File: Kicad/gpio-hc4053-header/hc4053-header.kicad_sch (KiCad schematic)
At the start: 7 parts, among them K1 GPIO IN, K2 I/O, K3 I/O, U1 74HC4053, U2 3M-SJ5376

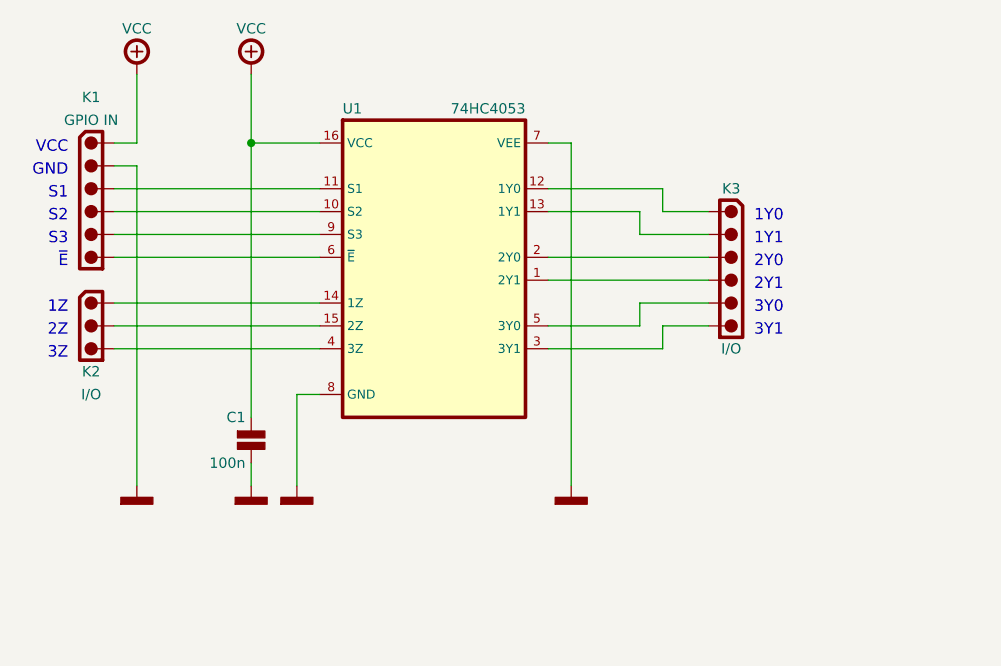
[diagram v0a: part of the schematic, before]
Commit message: Update
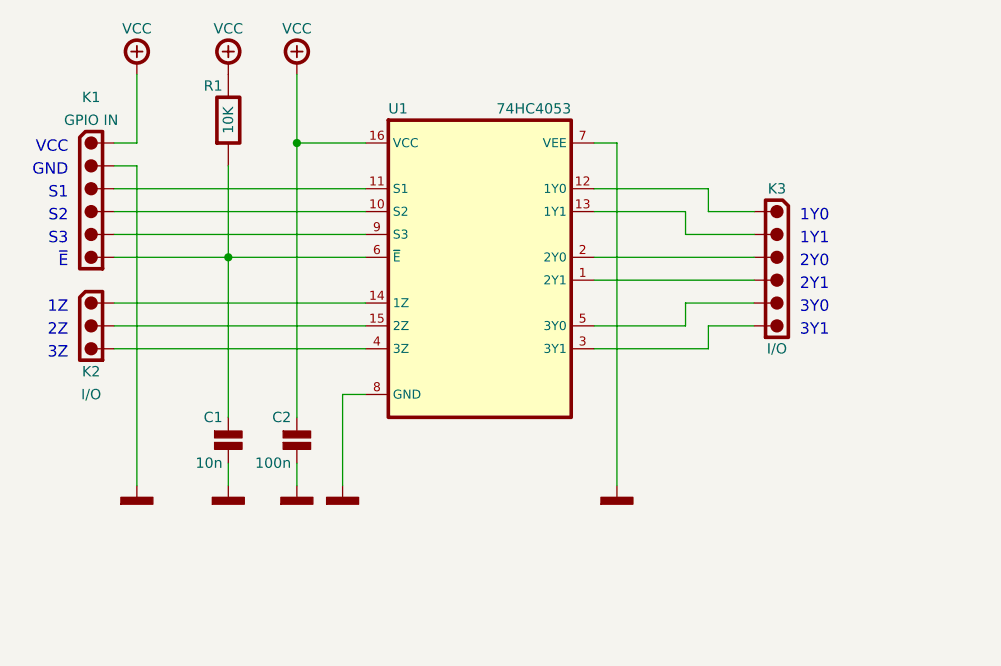
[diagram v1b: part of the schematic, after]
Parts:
- added C1: 10n, tronixio:CAPACITOR-SMD-1206, symbol tronixio:CAPACITOR-1206-10N
- added R1: 10K, tronixio:RESISTOR-SMD-1206, symbol tronixio:RESISTOR-1206-10K
- renumbered C1 to C2
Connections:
- net GND: now also C1.2
- net VCC: now also R1.1
- net at K1.6, U1.6 (~{E}): now also C1.1, R1.2
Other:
- moved on the sheet: C2, K3, U1
